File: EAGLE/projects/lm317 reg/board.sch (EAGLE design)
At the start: 1 part

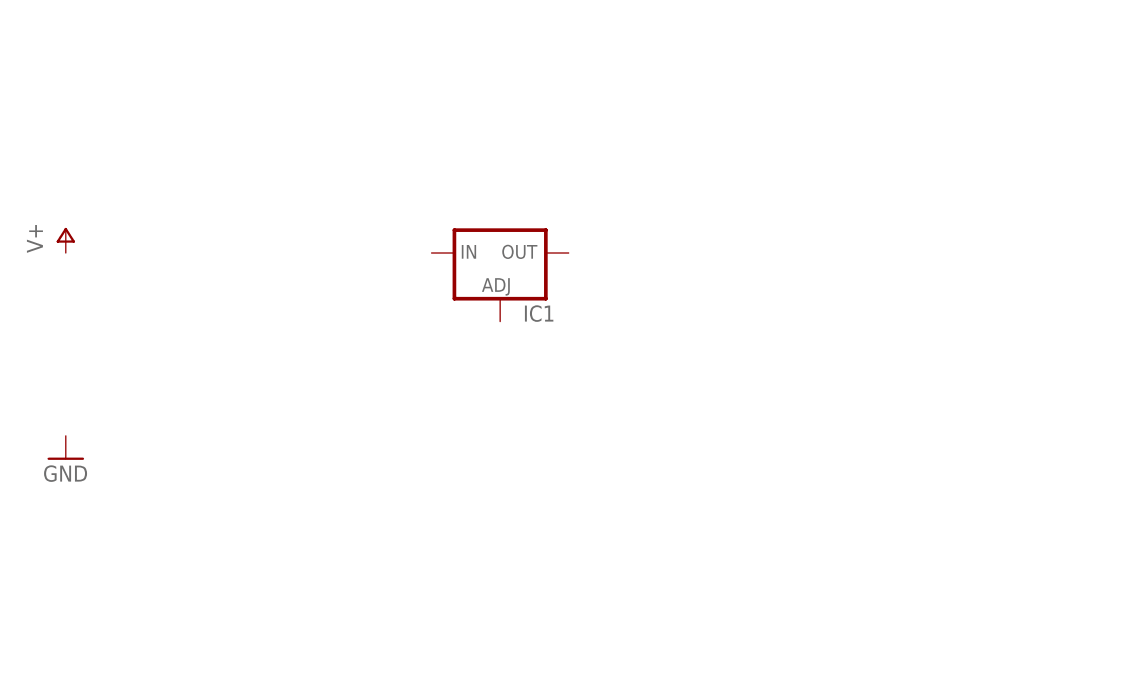
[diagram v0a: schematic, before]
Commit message: LM317 Reg
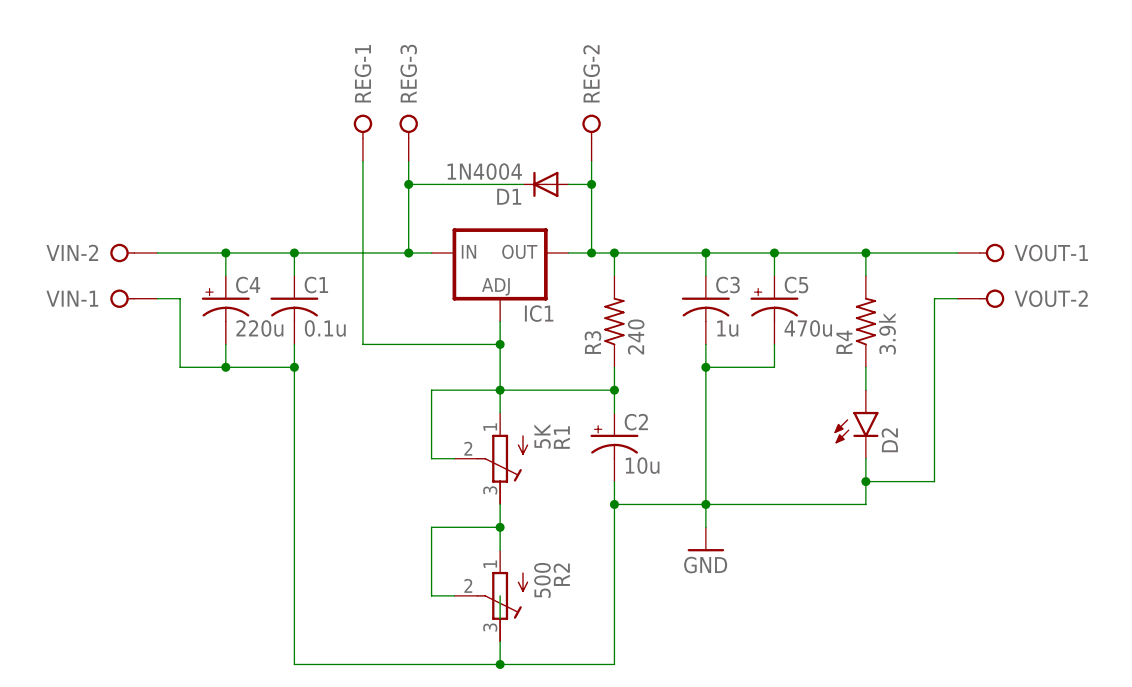
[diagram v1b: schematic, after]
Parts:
- added C1: 0.1u, rcl:C-USC1206
- added C2: 10u, rcl:CPOL-USE2-5
- added C3: 1u, rcl:C-USC1206
- added C4: 220u, rcl:CPOL-USE5-10.5
- added C5: 470u, rcl:CPOL-USE5-13
- added D1: 1N4004, diode:1N4004
- added D2: (no value), SparkFun-LED:LED1206
- added R1: 5K, rcl:R-TRIMM3296W
- added R2: 500, rcl:R-TRIMM3296W
- added R3: 240, rcl:R-US_0309/10
- added R4: 3.9k, rcl:R-US_R1206
- added REG: (no value), con-wago-508:W237-3E
- added VIN, VOUT: (no value), con-wago-508:W237-02P
- IC1: device v-reg:LM317-TO3 -> v-reg:LM317TS
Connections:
- new net GND: C1.2, C2.-, C3.2, C4.-, C5.-, D2.C, R2.E, VIN-1.KL, VOUT-2.KL
- new net N$1: C1.1, C4.+, D1.C, IC1.IN, REG-3.KL, VIN-2.KL
- new net N$2: D2.A, R4.1
- new net N$3: C2.+, IC1.ADJ, R1.A, R1.S, R3.1, REG-1.KL
- new net N$4: R1.E, R2.A, R2.S
- new net N$6: C3.1, C5.+, D1.A, IC1.OUT, R3.2, R4.2, REG-2.KL, VOUT-1.KL
